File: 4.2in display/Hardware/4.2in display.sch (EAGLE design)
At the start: 41 parts, among them J2 MICRO-SD_CARD_SOCKETPUSH-PUSH, Q1 310mA/60V/1.6Ω, U2 3.3V, U4 23K640

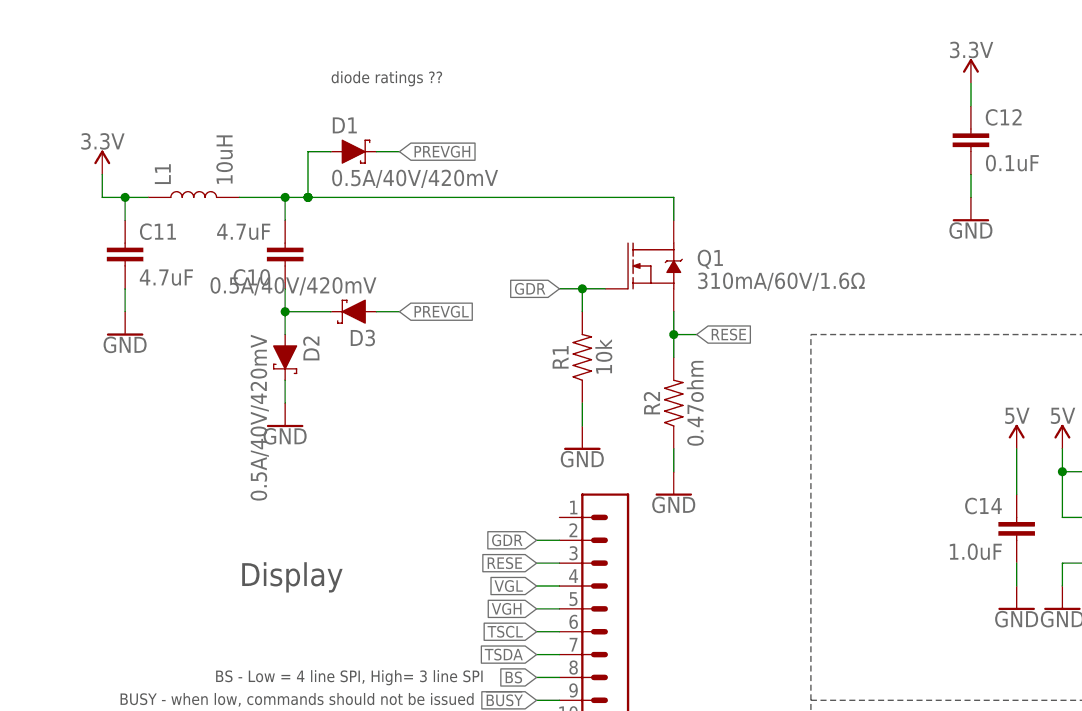
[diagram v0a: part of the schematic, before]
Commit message: Revert "Revert "asm""
This reverts commit b489ea2ff6e59cc2c3bae19cf3fe86e4ee51237d.
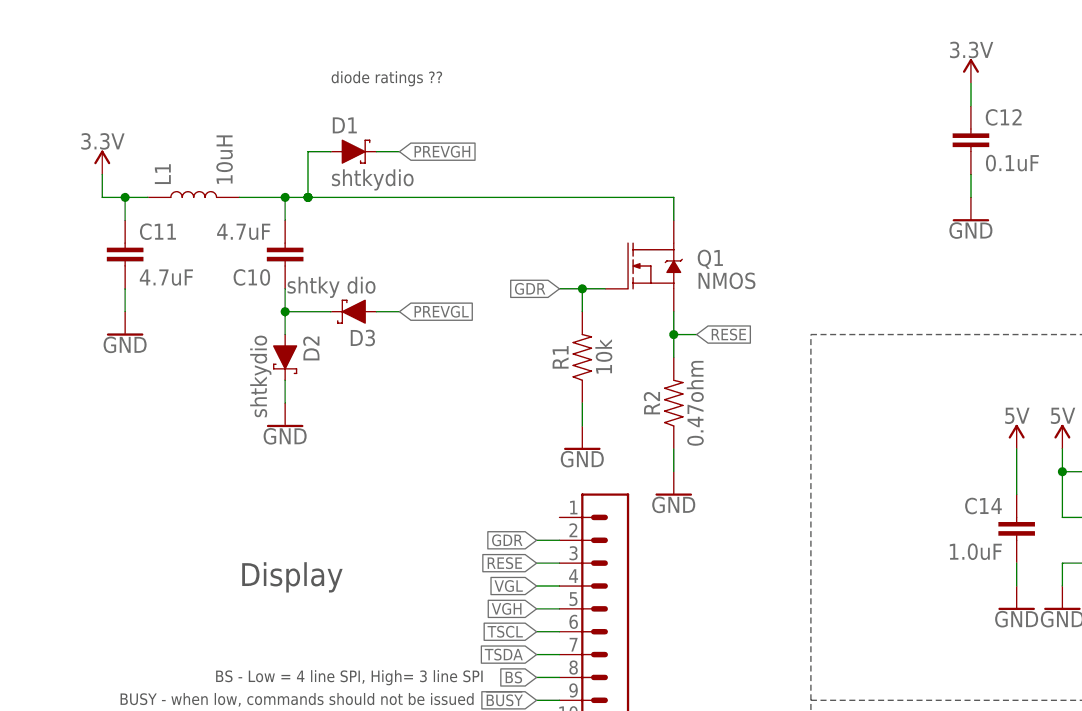
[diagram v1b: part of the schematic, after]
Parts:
- D1, D2: value 0.5A/40V/420mV -> shtkydio
- D3: value 0.5A/40V/420mV -> shtky dio
- Q1: value 310mA/60V/1.6Ω -> NMOS
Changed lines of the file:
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@@
 <part name="C8" library="SparkFun-Capacitors" deviceset="1.0UF" device="-0805-25V-10%" value="1.0uF"/>
 <part name="GND9" library="SparkFun-PowerSymbols" deviceset="GND" device=""/>
-<part name="Q1" library="SparkFun-DiscreteSemi" deviceset="MOSFET-NCH" device="-2N7002PW" value="310mA/60V/1.6Ω"/>
-<part name="D1" library="SparkFun-DiscreteSemi" deviceset="DIODE-SCHOTTKY" device="-PMEG4005EJ" value="0.5A/40V/420mV"/>
-<part name="D2" library="SparkFun-DiscreteSemi" deviceset="DIODE-SCHOTTKY" device="-PMEG4005EJ" value="0.5A/40V/420mV"/>
-<part name="D3" library="SparkFun-DiscreteSemi" deviceset="DIODE-SCHOTTKY" device="-PMEG4005EJ" value="0.5A/40V/420mV"/>
+<part name="Q1" library="SparkFun-DiscreteSemi" deviceset="MOSFET-NCH" device="-2N7002PW" value="NMOS"/>
+<part name="D1" library="SparkFun-DiscreteSemi" deviceset="DIODE-SCHOTTKY" device="-PMEG4005EJ" value="shtkydio"/>
+<part name="D2" library="SparkFun-DiscreteSemi" deviceset="DIODE-SCHOTTKY" device="-PMEG4005EJ" value="shtkydio"/>
+<part name="D3" library="SparkFun-DiscreteSemi" deviceset="DIODE-SCHOTTKY" device="-PMEG4005EJ" value="shtky dio"/>
 <part name="C9" library="SparkFun-Capacitors" deviceset="1.0UF" device="-0805-25V-10%" value="1.0uF"/>
 <part name="GND10" library="SparkFun-PowerSymbols" deviceset="GND" device=""/>

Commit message: Revert "Revert "Revert "asm"""
This reverts commit 13aa5e244575f702f785403d246ecc40f8071a55.
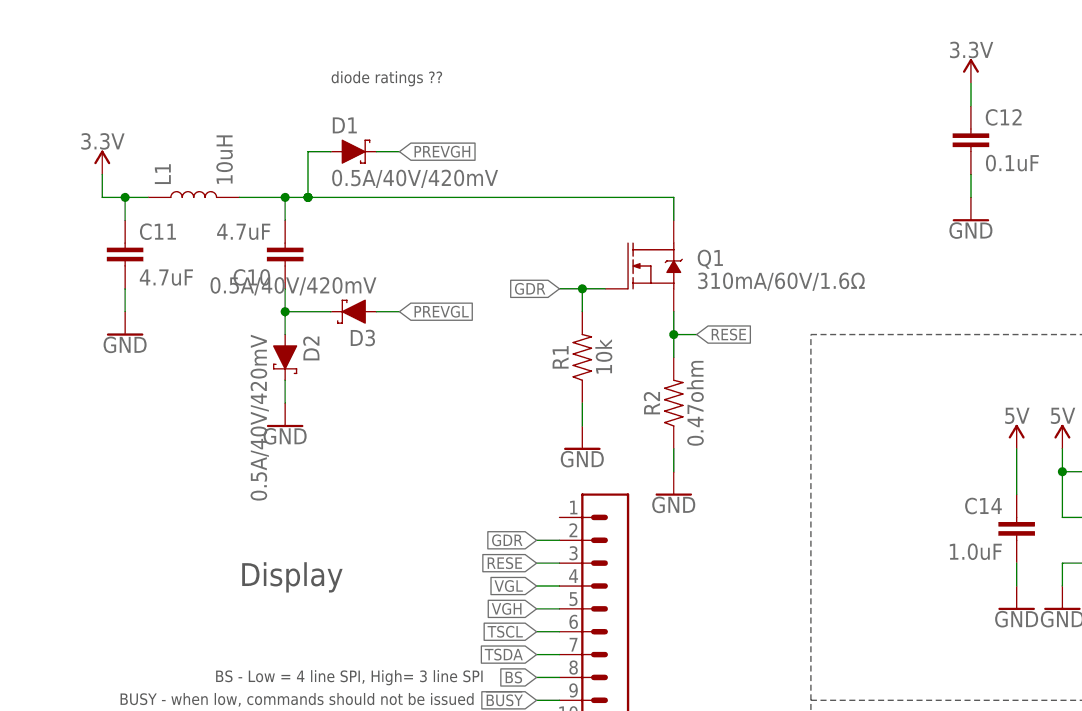
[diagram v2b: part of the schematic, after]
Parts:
- D1, D2: value shtkydio -> 0.5A/40V/420mV
- D3: value shtky dio -> 0.5A/40V/420mV
- Q1: value NMOS -> 310mA/60V/1.6Ω
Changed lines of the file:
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@@
 <part name="C8" library="SparkFun-Capacitors" deviceset="1.0UF" device="-0805-25V-10%" value="1.0uF"/>
 <part name="GND9" library="SparkFun-PowerSymbols" deviceset="GND" device=""/>
-<part name="Q1" library="SparkFun-DiscreteSemi" deviceset="MOSFET-NCH" device="-2N7002PW" value="NMOS"/>
-<part name="D1" library="SparkFun-DiscreteSemi" deviceset="DIODE-SCHOTTKY" device="-PMEG4005EJ" value="shtkydio"/>
-<part name="D2" library="SparkFun-DiscreteSemi" deviceset="DIODE-SCHOTTKY" device="-PMEG4005EJ" value="shtkydio"/>
-<part name="D3" library="SparkFun-DiscreteSemi" deviceset="DIODE-SCHOTTKY" device="-PMEG4005EJ" value="shtky dio"/>
+<part name="Q1" library="SparkFun-DiscreteSemi" deviceset="MOSFET-NCH" device="-2N7002PW" value="310mA/60V/1.6Ω"/>
+<part name="D1" library="SparkFun-DiscreteSemi" deviceset="DIODE-SCHOTTKY" device="-PMEG4005EJ" value="0.5A/40V/420mV"/>
+<part name="D2" library="SparkFun-DiscreteSemi" deviceset="DIODE-SCHOTTKY" device="-PMEG4005EJ" value="0.5A/40V/420mV"/>
+<part name="D3" library="SparkFun-DiscreteSemi" deviceset="DIODE-SCHOTTKY" device="-PMEG4005EJ" value="0.5A/40V/420mV"/>
 <part name="C9" library="SparkFun-Capacitors" deviceset="1.0UF" device="-0805-25V-10%" value="1.0uF"/>
 <part name="GND10" library="SparkFun-PowerSymbols" deviceset="GND" device=""/>

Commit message: Revert "sch"
This reverts commit 65ffcdcff918ffc3cbfeebb47afa4d674ba5142f.
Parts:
- C1: value 1.0uF -> 1.0uF
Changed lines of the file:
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@@
 <?xml version="1.0" encoding="utf-8"?>
 <!DOCTYPE eagle SYSTEM "eagle.dtd">
-<eagle version="9.1.3">
+<eagle version="9.0.1">
 <drawing>
 <settings>
@@
 <part name="U$1" library="ePaper" deviceset="24_PIN_FPC_0.5MM" device=""/>
 <part name="GND1" library="SparkFun-PowerSymbols" deviceset="GND" device=""/>
-<part name="C1" library="SparkFun-Capacitors" deviceset="1.0UF" device="-0603-16V-10%" value="1.0uF "/>
+<part name="C1" library="SparkFun-Capacitors" deviceset="1.0UF" device="-0603-16V-10%" value="1.0uF"/>
 <part name="C2" library="SparkFun-Capacitors" deviceset="1.0UF" device="-0805-25V-10%" value="1.0uF"/>
 <part name="C3" library="SparkFun-Capacitors" deviceset="1.0UF" device="-0805-25V-10%" value="1.0uF"/>

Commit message: sch
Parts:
- C1: value 1.0uF -> 1.0uF
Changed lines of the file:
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@@
 <?xml version="1.0" encoding="utf-8"?>
 <!DOCTYPE eagle SYSTEM "eagle.dtd">
-<eagle version="9.0.1">
+<eagle version="9.1.3">
 <drawing>
 <settings>
@@
 <part name="U$1" library="ePaper" deviceset="24_PIN_FPC_0.5MM" device=""/>
 <part name="GND1" library="SparkFun-PowerSymbols" deviceset="GND" device=""/>
-<part name="C1" library="SparkFun-Capacitors" deviceset="1.0UF" device="-0603-16V-10%" value="1.0uF"/>
+<part name="C1" library="SparkFun-Capacitors" deviceset="1.0UF" device="-0603-16V-10%" value="1.0uF "/>
 <part name="C2" library="SparkFun-Capacitors" deviceset="1.0UF" device="-0805-25V-10%" value="1.0uF"/>
 <part name="C3" library="SparkFun-Capacitors" deviceset="1.0UF" device="-0805-25V-10%" value="1.0uF"/>
